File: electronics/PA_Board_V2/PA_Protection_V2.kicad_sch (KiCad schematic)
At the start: 61 parts, among them J10 Conn_01x05, J2 Conn_01x04, J3 Conn_01x05, J6 Conn_01x06, J9 USB_B_Micro, SW1 SW_Push, U12 LM2904, U13 ATSAMD21E18A-A, U15 74LV1T34, U2 LM75B, U5 74LV1T34

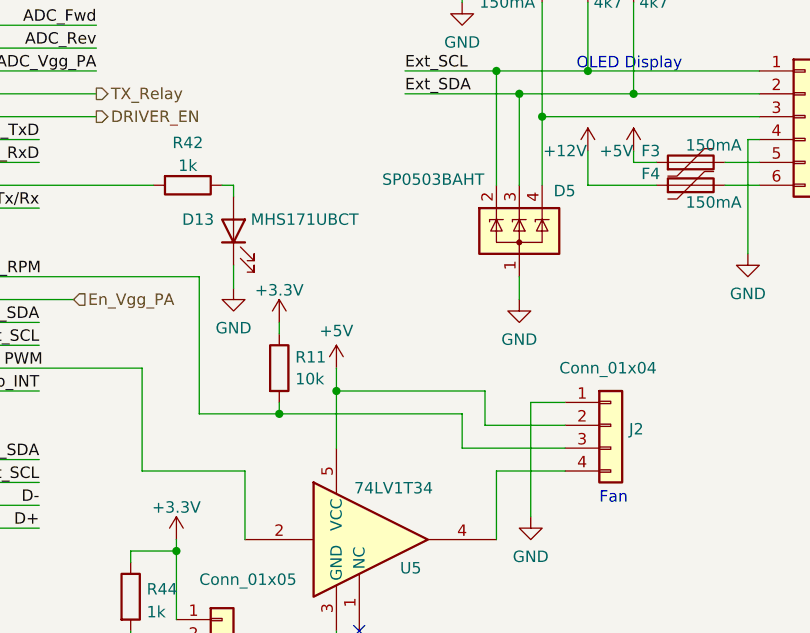
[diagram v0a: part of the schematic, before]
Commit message: Updates in electronics bits and bobs
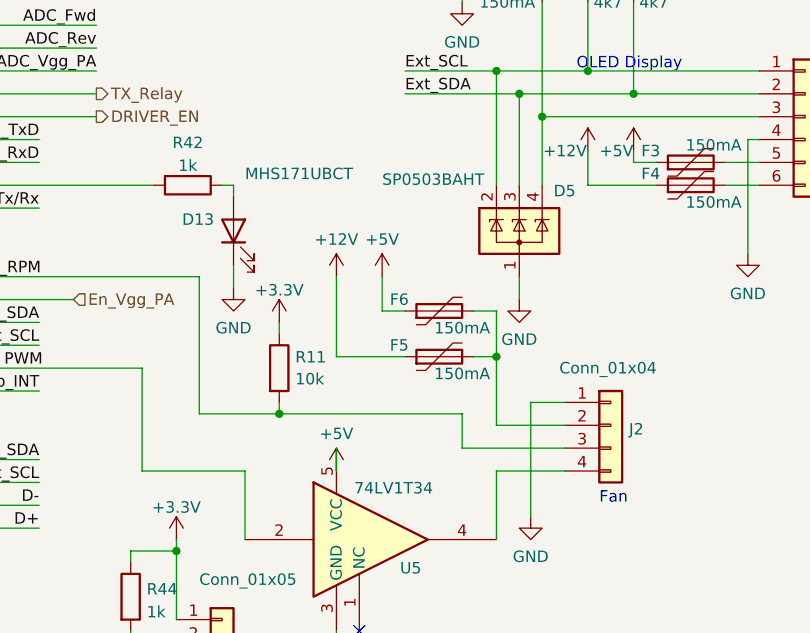
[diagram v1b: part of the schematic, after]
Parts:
- added F5, F6: 150mA, Fuse:Fuse_0805_2012Metric, symbol Device:Polyfuse
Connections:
- net +12V: now also F5.1
- net +5V: now also F6.1; no longer J2.2 (Pin_2)
- new net: F5.2, F6.2, J2.2 (Pin_2)
